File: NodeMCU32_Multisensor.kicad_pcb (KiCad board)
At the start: 2 copper layers, 32 parts, among them J1 DHT22, J2 LED, J3 PIR Sensor (HC-SR505), J4 Feuchtesensor, J5 Pumpe, J6 Screw_Terminal_01x02, J7 Conn_01x05_Male, J8 Conn_01x04_Male, K1 SRD-05VDC-SL-C, Q1 BC547, U1 ESP32-DEVKITC-32D, U2 HC-SR04

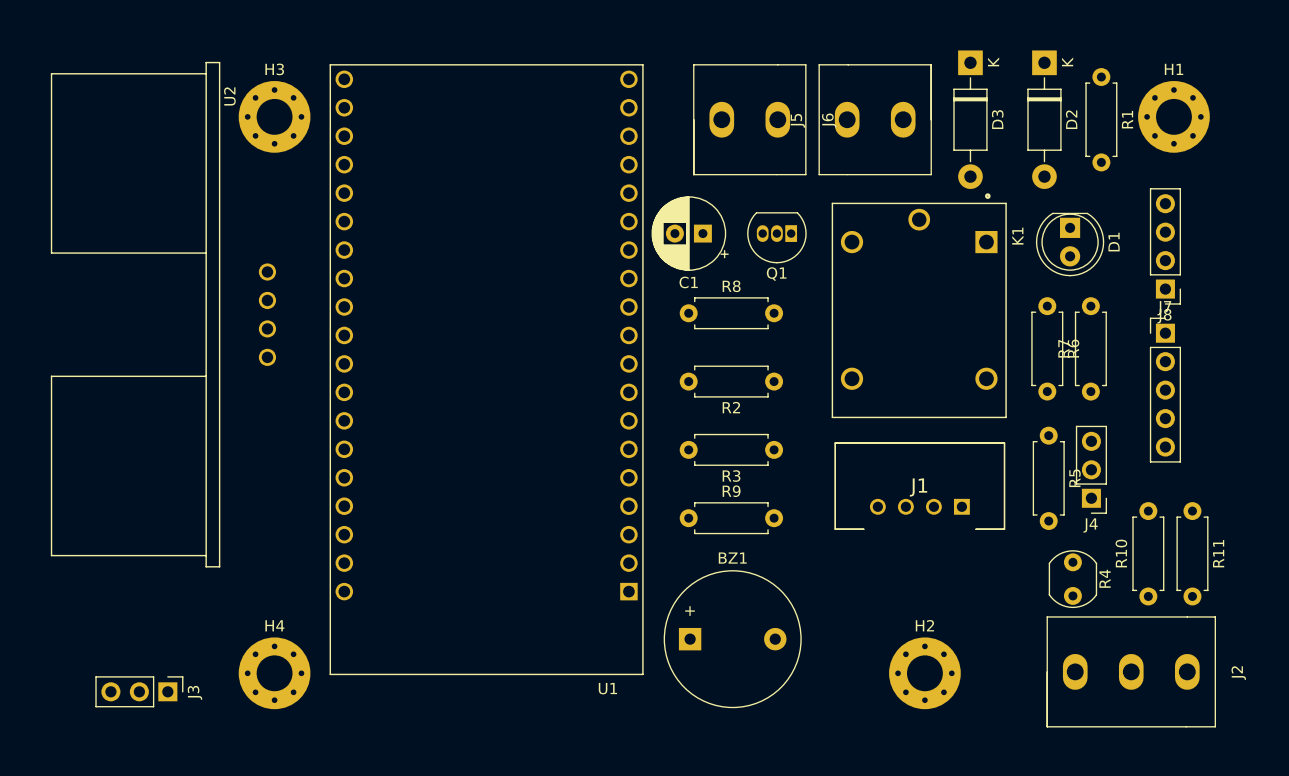
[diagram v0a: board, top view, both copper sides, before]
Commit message: finished pcb layout. check needed.
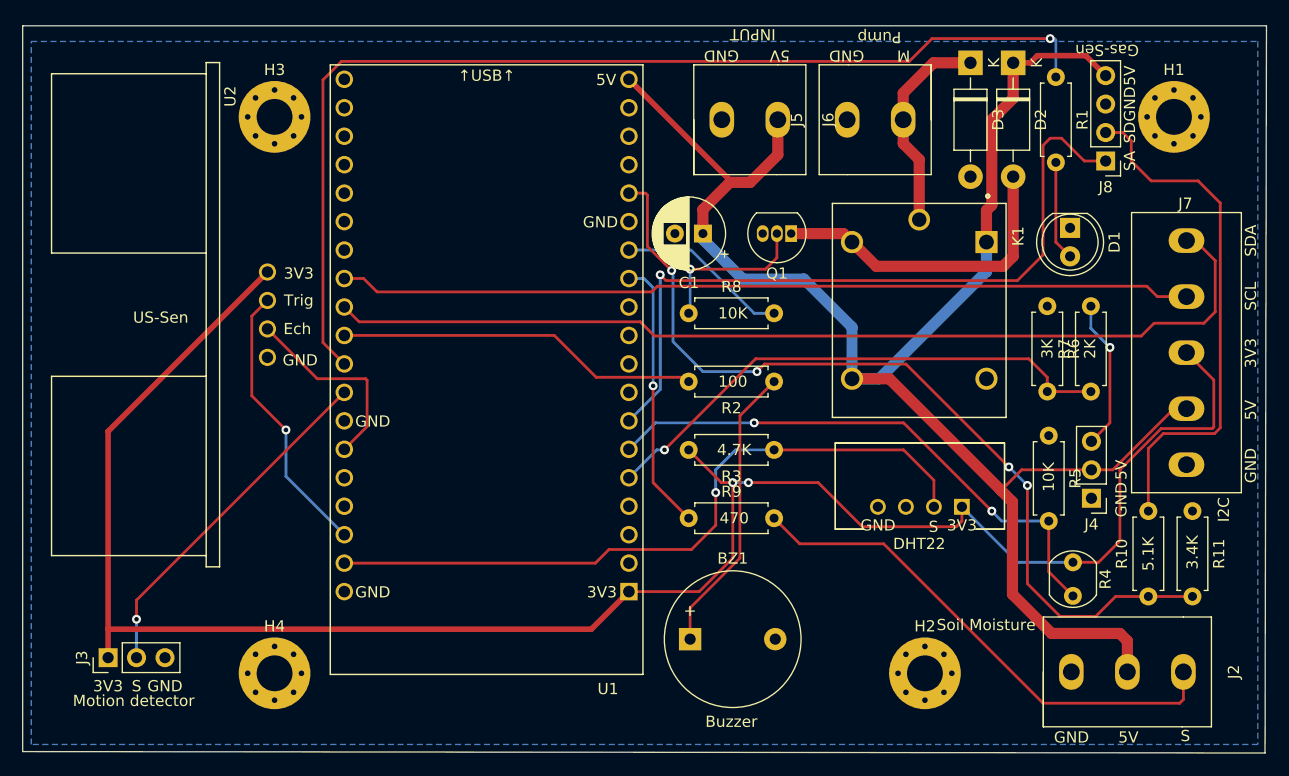
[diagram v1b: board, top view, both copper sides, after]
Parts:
- J7: footprint Connector_PinHeader_2.54mm:PinHeader_1x05_P2.54mm_Vertical -> TerminalBlock:ScrewTerminal_1x5_P5.00
- moved J8 12.6 mm to (142.9, 69.7)
- moved J7 12.2 mm to (150.0, 73.0)
- moved J3 6.14 mm to (53.8, 114.0), turned to 90 degrees
- moved R1 4.06 mm to (138.4, 62.2)
- moved D2 2.79 mm to (134.6, 61.0)
- moved J2 0.35 mm to (154.8, 115.3)
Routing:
- net +3V3: track 0.00 -> 175.0 mm, vias 0 -> 2
- net +5V: track 0.00 -> 154.9 mm
- net ESP.18-LED: track 0.00 -> 96.4 mm, vias 0 -> 1
- net ESP.17-SDA: track 0.00 -> 87.6 mm
- net ESP.13-DigGas: track 0.00 -> 78.7 mm, vias 0 -> 4
- net ESP.16-SCL: track 0.00 -> 76.2 mm
- net ESP.32-AnaGas: track 0.00 -> 66.0 mm, vias 0 -> 1
- net ESP.23-DHT22: track 0.00 -> 63.2 mm, vias 0 -> 1
- net ESP.35-Helligkeitssensor: track 0.00 -> 49.6 mm, vias 0 -> 2
- net ESP.34-Feuchtesensor: track 0.00 -> 47.6 mm, vias 0 -> 1
- net Net-(J8-Pad2): track 0.00 -> 46.7 mm
- net Net-(J2-Pad1): track 0.00 -> 46.7 mm
- net ESP.5-Buzzer: track 0.00 -> 32.4 mm
- net ESP.19-Bewegungsmelder: track 0.00 -> 31.4 mm, vias 0 -> 1
- net Net-(D2-Pad2): track 0.00 -> 28.5 mm
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- added copper zone on B.Cu, net GND
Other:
- board outline added: 111 x 64.9 mm
- board text added: "100"
- board text added: "10K"
- board text added: "2K"
- board text added: "3.4K"
- board text added: "3K"
- board text added: "3V3"
- board text added: "4.7K"
- board text added: "470"
- board text added: "5.1K"
- board text added: "5V"
- board text added: "Buzzer"
- board text added: "DHT22"
- board text added: "Designed by Dirk & Björn Ellwert"
- board text added: "Ech"
- board text added: "GND"
- board text added: "Gas-Sen"
- board text added: "I2C"
- board text added: "INPUT"
- board text added: "M"
- board text added: "Motion detector"
- board text added: "Pump"
- board text added: "S"
- board text added: "SA"
- board text added: "SCL"
- board text added: "SD"
- board text added: "SDA"
- board text added: "Soil Moisture"
- board text added: "Trig"
- board text added: "US-Sen"
- board text added: "↑USB↑"
